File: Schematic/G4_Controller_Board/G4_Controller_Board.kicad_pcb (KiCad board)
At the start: 2 copper layers, 124.5 x 36.8 mm, 39 parts, among them J10 Solenoid, J11 Inter-board Jumper, J12 Inter-board Jumper, J15 IR LED Rec., J16 IR LED Emitter, J17 Positive BUS, J18 Negative BUS, J2 ESC Right, J3 ESC Left, J6 Rev Trigger (Optional), J7 Fire Trigger, J8 Magazine Removal Trigger, J9 I2C Out, Q1 2N7000, Q2 Q_NMOS_GDS, Q3 Q_PMOS_GDS, SW2 Preset A, SW3 Preset B, SW4 Preset C, SW7 RotaryEncoder_Switch, U1 ESP32-LOLIN32-Lite, U2 Mini360

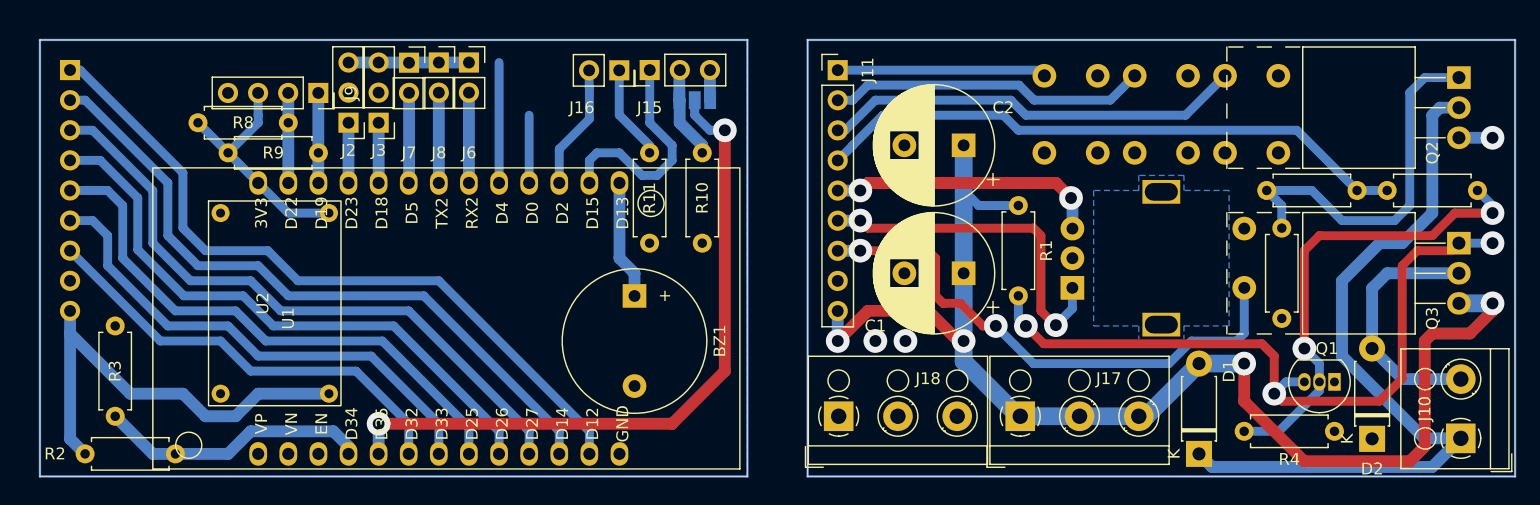
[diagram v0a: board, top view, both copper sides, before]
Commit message: update PCB
prototype revision should be completed
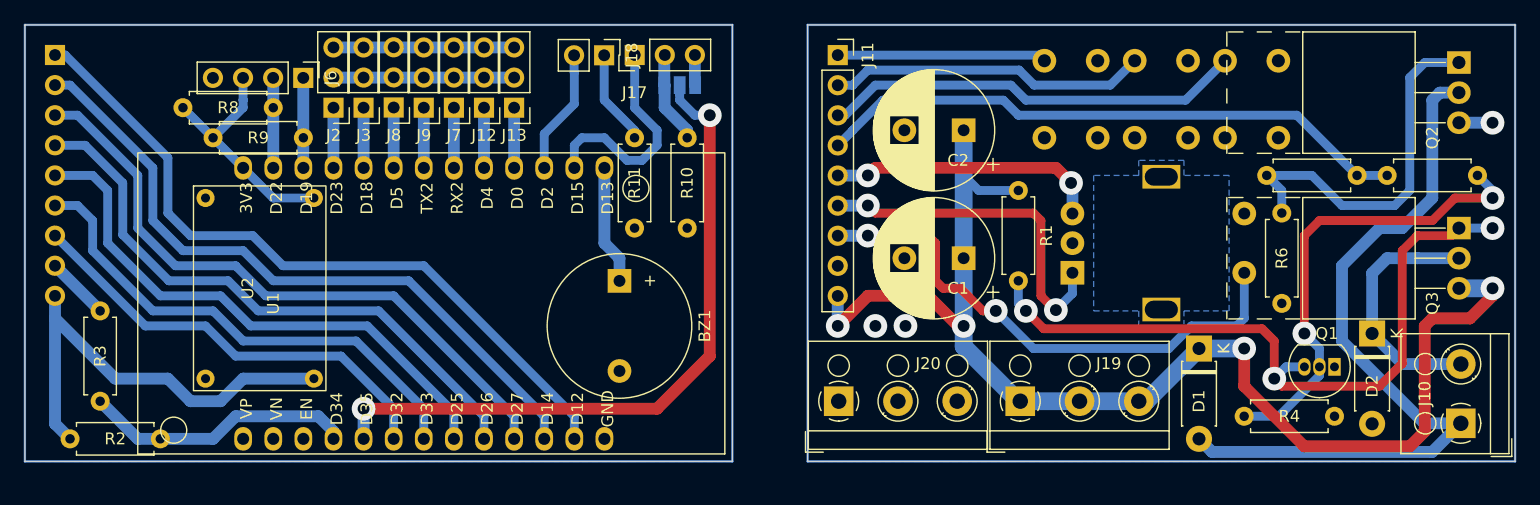
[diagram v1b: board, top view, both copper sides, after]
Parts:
- removed the J6 at (92.1, 73.0)
- added J12: SolenoidTrig A (Optional), Connector_PinHeader_2.54mm:PinHeader_1x03_P2.54mm_Vertical, F.Cu at (93.3, 76.8)
- added J13: SolenoidTrig B (Optional), Connector_PinHeader_2.54mm:PinHeader_1x03_P2.54mm_Vertical, F.Cu at (95.9, 76.8)
- added J9: Magazine Removal Trigger, Connector_PinHeader_2.54mm:PinHeader_1x03_P2.54mm_Vertical, F.Cu at (88.3, 76.8)
- D1, D2: value DIODE -> 1N4001
- J11: value Inter-board Jumper -> Board Interconnect; footprint Connector_PinHeader_2.54mm:PinHeader_1x09_P2.54mm_Vertical -> Connector_PinSocket_2.54mm:PinSocket_1x09_P2.54mm_Vertical
- J14: renamed from J12; value Inter-board Jumper -> Board Interconnect; footprint Connector_PinSocket_2.54mm:PinSocket_1x09_P2.54mm_Vertical -> Connector_PinHeader_2.54mm:PinHeader_1x09_P2.54mm_Vertical
- J18: renamed from J16; footprint Connector_PinSocket_2.54mm:PinSocket_1x02_P2.54mm_Vertical -> Connector_PinHeader_2.54mm:PinHeader_1x02_P2.54mm_Vertical
- J6: renamed from J9; footprint Connector_PinSocket_2.54mm:PinSocket_1x04_P2.54mm_Vertical -> Connector_PinHeader_2.54mm:PinHeader_1x04_P2.54mm_Vertical
- J7: value Fire Trigger -> Rev Trigger (Optional); footprint Connector_PinSocket_2.54mm:PinSocket_1x02_P2.54mm_Vertical -> Connector_PinHeader_2.54mm:PinHeader_1x03_P2.54mm_Vertical
- J8: value Magazine Removal Trigger -> Fire Trigger; footprint Connector_PinSocket_2.54mm:PinSocket_1x02_P2.54mm_Vertical -> Connector_PinHeader_2.54mm:PinHeader_1x03_P2.54mm_Vertical
- moved D1 8.89 mm to (153.7, 97.2), turned to -90 degrees
- moved D2 8.89 mm to (168.3, 95.9), turned to -90 degrees
- moved J8 5.38 mm to (85.7, 76.8), turned to 180 degrees
- moved J7 5.36 mm to (90.8, 76.8), turned to 180 degrees
- moved J2 1.80 mm to (80.6, 76.8)
- moved R8 1.80 mm to (67.9, 76.8)
- moved J3 1.80 mm to (83.2, 76.8)
- moved J6 1.80 mm to (78.1, 74.3)
- moved R10 1.80 mm to (110.5, 87.0)
- moved J14 1.80 mm to (57.1, 72.4)
- moved BZ1 1.80 mm to (104.8, 91.5)
- moved J17 1.80 mm to (106.1, 72.4)
- moved J18 1.80 mm to (103.5, 72.4)
- moved JP1 1.80 mm to (109.9, 74.9)
- moved R11 1.80 mm to (106.0, 87.0)
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- renumbered J15 to J17, J17 to J19, J18 to J20
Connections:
- D1 pad 1: /SOLENOID_A -> +12V
- D1 pad 2: +12V -> /SOLENOID_A
- D2 pad 1: GND -> /SOLENOID_B
- D2 pad 2: /SOLENOID_B -> GND
- J2 pad 2: unconnected-(J2-Pin_2-Pad2) -> GND
- J3 pad 2: unconnected-(J3-Pin_2-Pad2) -> GND
- J7 pad 1: GND -> /RevTrg
- J7 pad 2: /FireTrg -> GND
- J8 pad 1: GND -> /FireTrg
- J8 pad 2: /MagTrg -> GND
- SW7 pad MP: (no net) -> Tab
- U1 pad 23: /SolenoidTrig B -> /SolTrig B
- U1 pad 24: /SolenoidTrig A -> /SolTrig A
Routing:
- net GND: track 13.0 -> 38.7 mm
- net /SolenoidTrig A: track 10.2 -> 0.00 mm
- net /SolenoidTrig B: track 5.72 -> 0.00 mm
- net /SolTrig B: track 0.00 -> 5.08 mm
- net /SolTrig A: track 0.00 -> 5.08 mm
- net /RevTrg: track 7.62 -> 5.08 mm
- net /MagTrg: track 7.62 -> 5.08 mm
- net /FireTrg: track 7.61 -> 5.12 mm
- net Tab: track 0.00 -> 0.90 mm
- net (no net): track 0.90 -> 0.00 mm
- added copper zone on B.Cu, net Tab
- removed copper zone on B.Cu, net (none)
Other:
- board size 124.5 x 36.8 mm -> 125.7 x 36.8 mm
